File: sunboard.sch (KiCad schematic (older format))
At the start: 25 parts, among them J1 Conn_01x04, J2 Conn_01x02, J3 Barrel_Jack, J4 Conn_01x04, SW1 SW_Push, U1 STM32F030C8Tx, U4 MIC5209, Y1 Crystal_Small

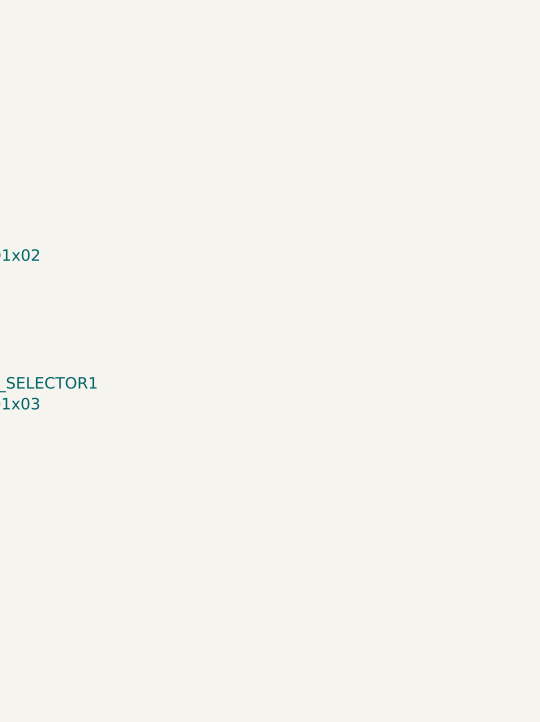
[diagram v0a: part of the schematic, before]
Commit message: init change lc branch
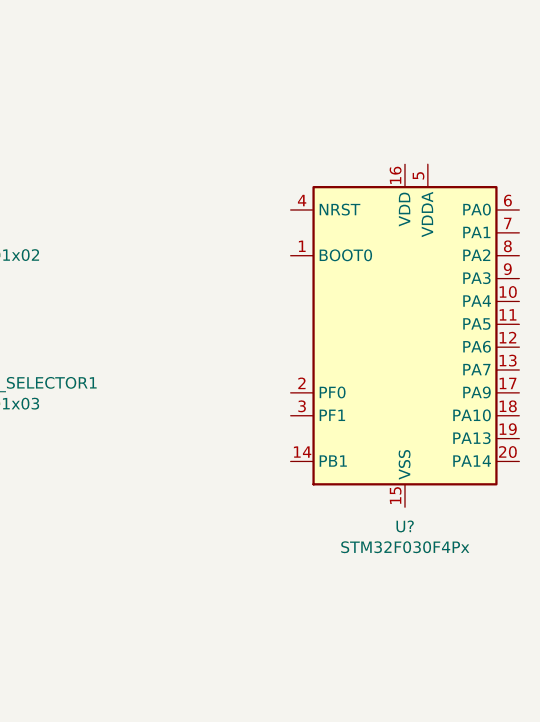
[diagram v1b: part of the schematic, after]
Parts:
- added U?: STM32F030F4Px, Package_SO:TSSOP-20_4.4x6.5mm_P0.65mm, symbol MCU_ST_STM32F0:STM32F030F4Px
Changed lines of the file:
@@
 Text Label 4150 6600 0    50   ~ 0
 SWDIO
+$Comp
+L MCU_ST_STM32F0:STM32F030F4Px U?
+U 1 1 5C6A2359
+P 8850 4000
+F 0 "U?" H 8850 3114 50  0000 C CNN
+F 1 "STM32F030F4Px" H 8850 3023 50  0000 C CNN
+F 2 "Package_SO:TSSOP-20_4.4x6.5mm_P0.65mm" H 8450 3300 50  0001 R CNN
+F 3 "http://www.st.com/st-web-ui/static/active/en/resource/technical/document/datasheet/DM00088500.pdf" H 8850 4000 50  0001 C CNN
+	1    8850 4000
+	1    0    0    -1
+$EndComp
 $EndSCHEMATC

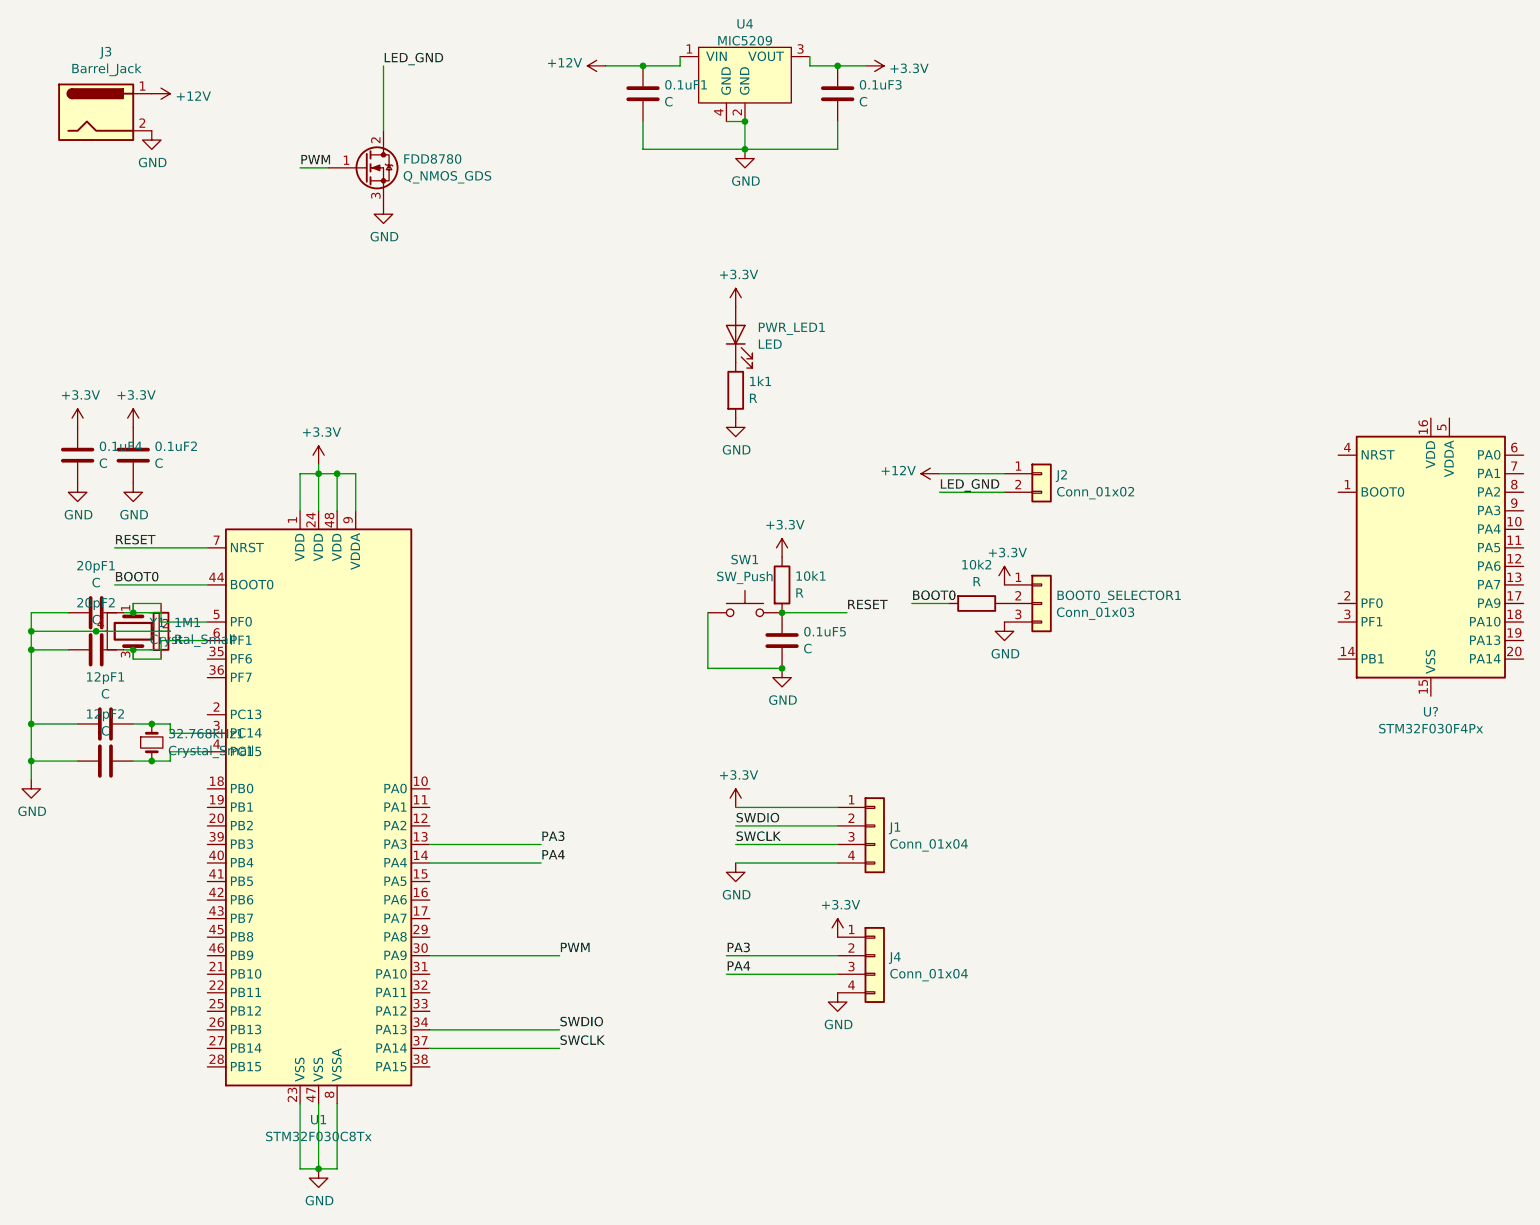
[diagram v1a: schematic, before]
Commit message: updated sch and pcb
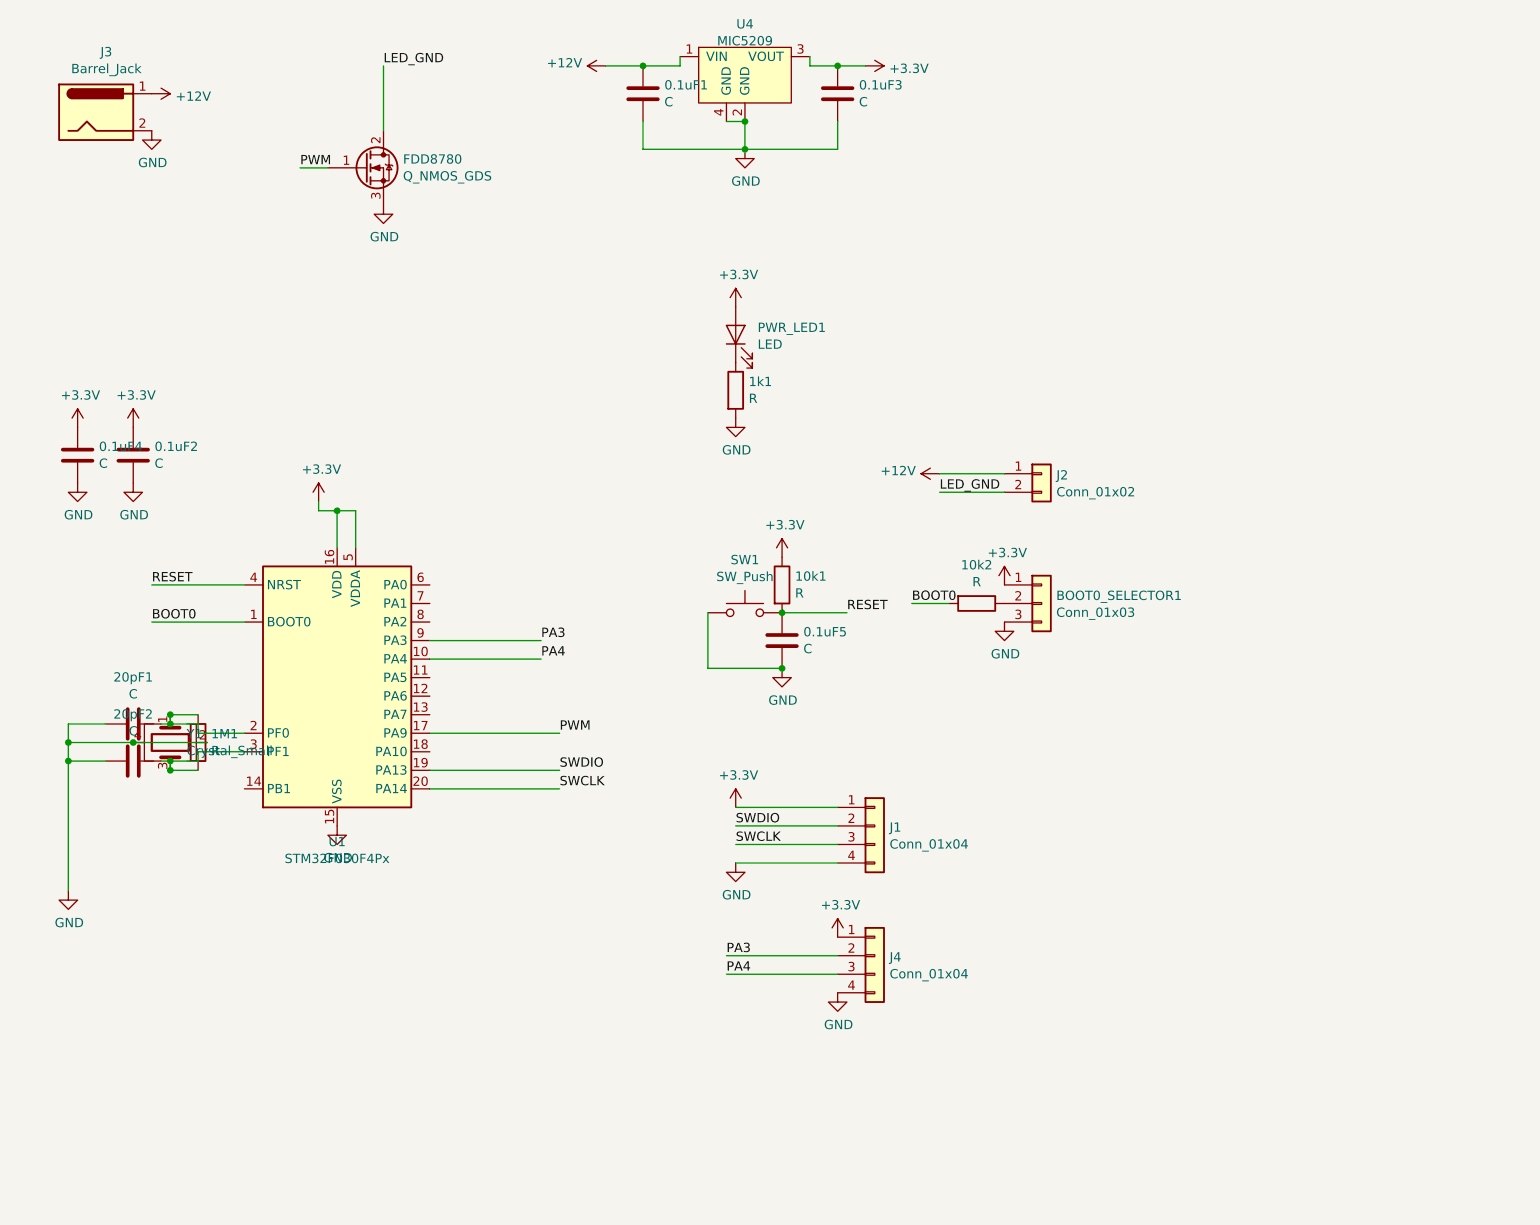
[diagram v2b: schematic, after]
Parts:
- removed 12pF1, 12pF2: C, Capacitor_SMD:C_0603_1608Metric, symbol Device:C
- removed 32.768kHz1: Crystal_Small, Crystal:Crystal_SMD_3215-2Pin_3.2x1.5mm, symbol Device:Crystal_Small
- removed U1: STM32F030C8Tx, Package_QFP:LQFP-48_7x7mm_P0.5mm, symbol MCU_ST_STM32F0:STM32F030C8Tx
- gave numbers to parts that had none: 1
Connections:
- net +3V3: now also U1.16 (VDD), U1.5 (VDDA)
- net BOOT0: now also U1.1 (BOOT0)
- net GND: now also U1.15 (VSS)
- net PA3: now also U1.9 (PA3)
- net PA4: now also U1.10 (PA4)
- net PWM: now also U1.17 (PA9)
- net RESET: now also U1.4 (NRST)
- net SWCLK: now also U1.20 (PA14)
- net SWDIO: now also U1.19 (PA13)
- net at 1M1.1, 20pF1.1, Y1.1: now also U1.2 (PF0)
- net at 1M1.2, 20pF2.1, Y1.3: now also U1.3 (PF1)
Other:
- moved on the sheet: 1M1, 20pF1, 20pF2, U1, Y1
